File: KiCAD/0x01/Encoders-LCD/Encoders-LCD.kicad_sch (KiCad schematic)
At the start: 32 parts, among them J1 Conn_01x04, J2 Conn_01x04, SW1 SW_LEFT, SW2 SW_SHIFT, SW3 SW_RIGHT, U1 ATtiny412-SS, U2 3631AS, U3 3631AS, U4 ATtiny412-SS, U5 HT16K33 24SOP, U6 ATtiny412-SS

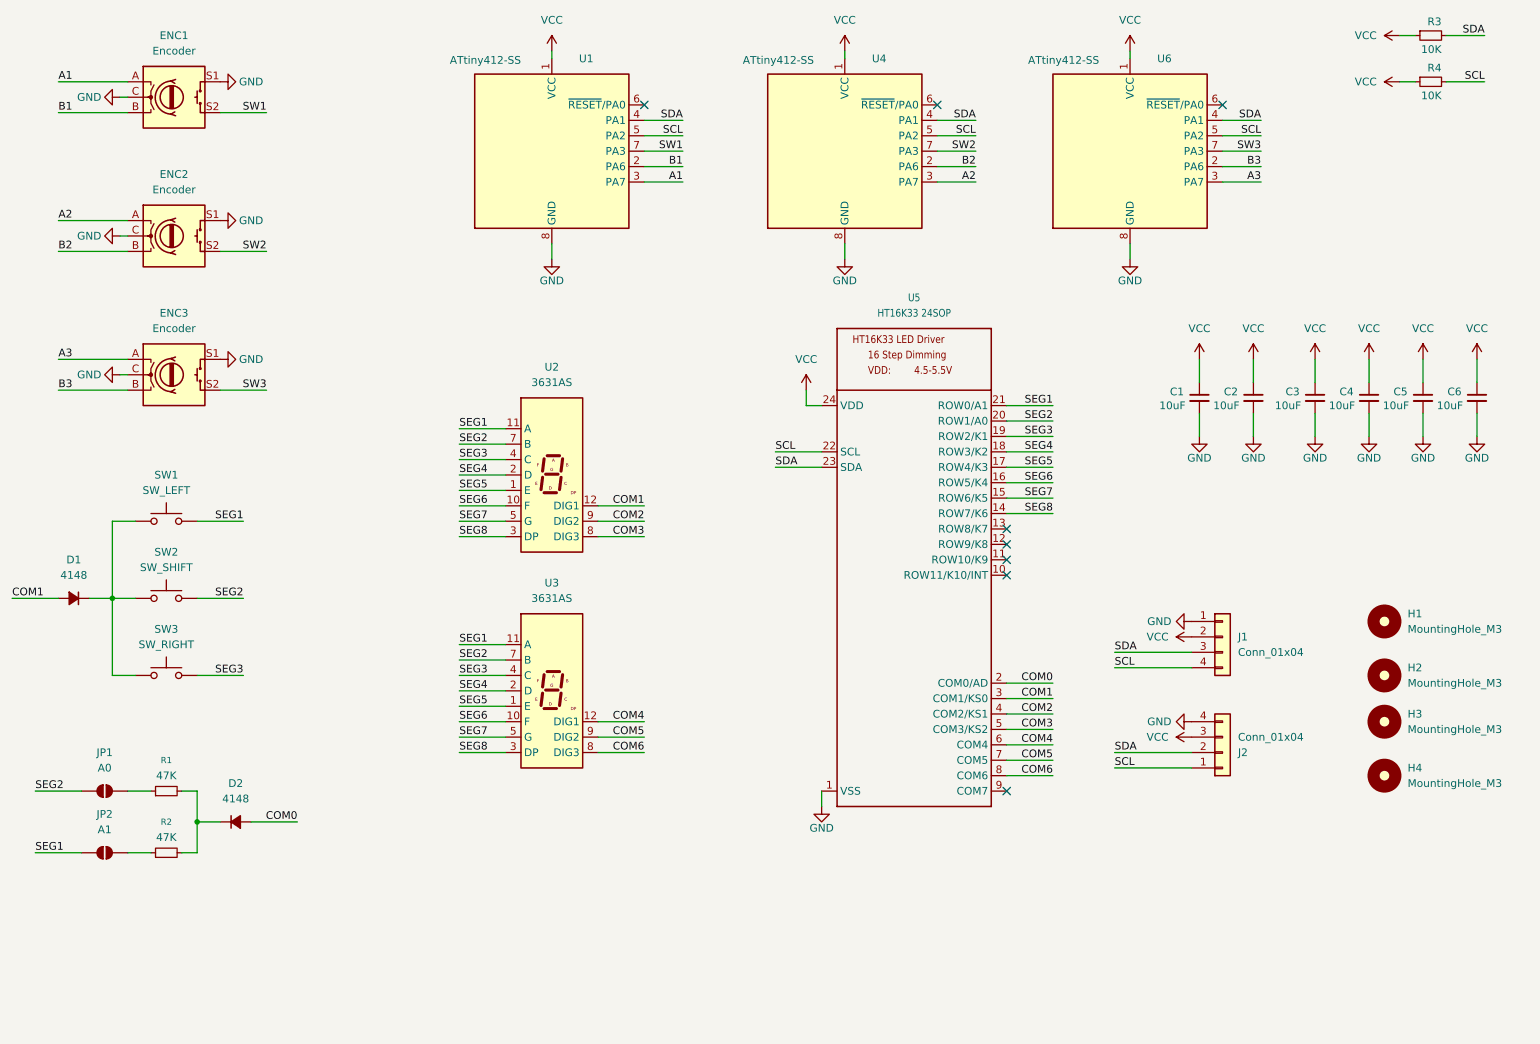
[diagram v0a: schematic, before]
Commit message: lcd encoders
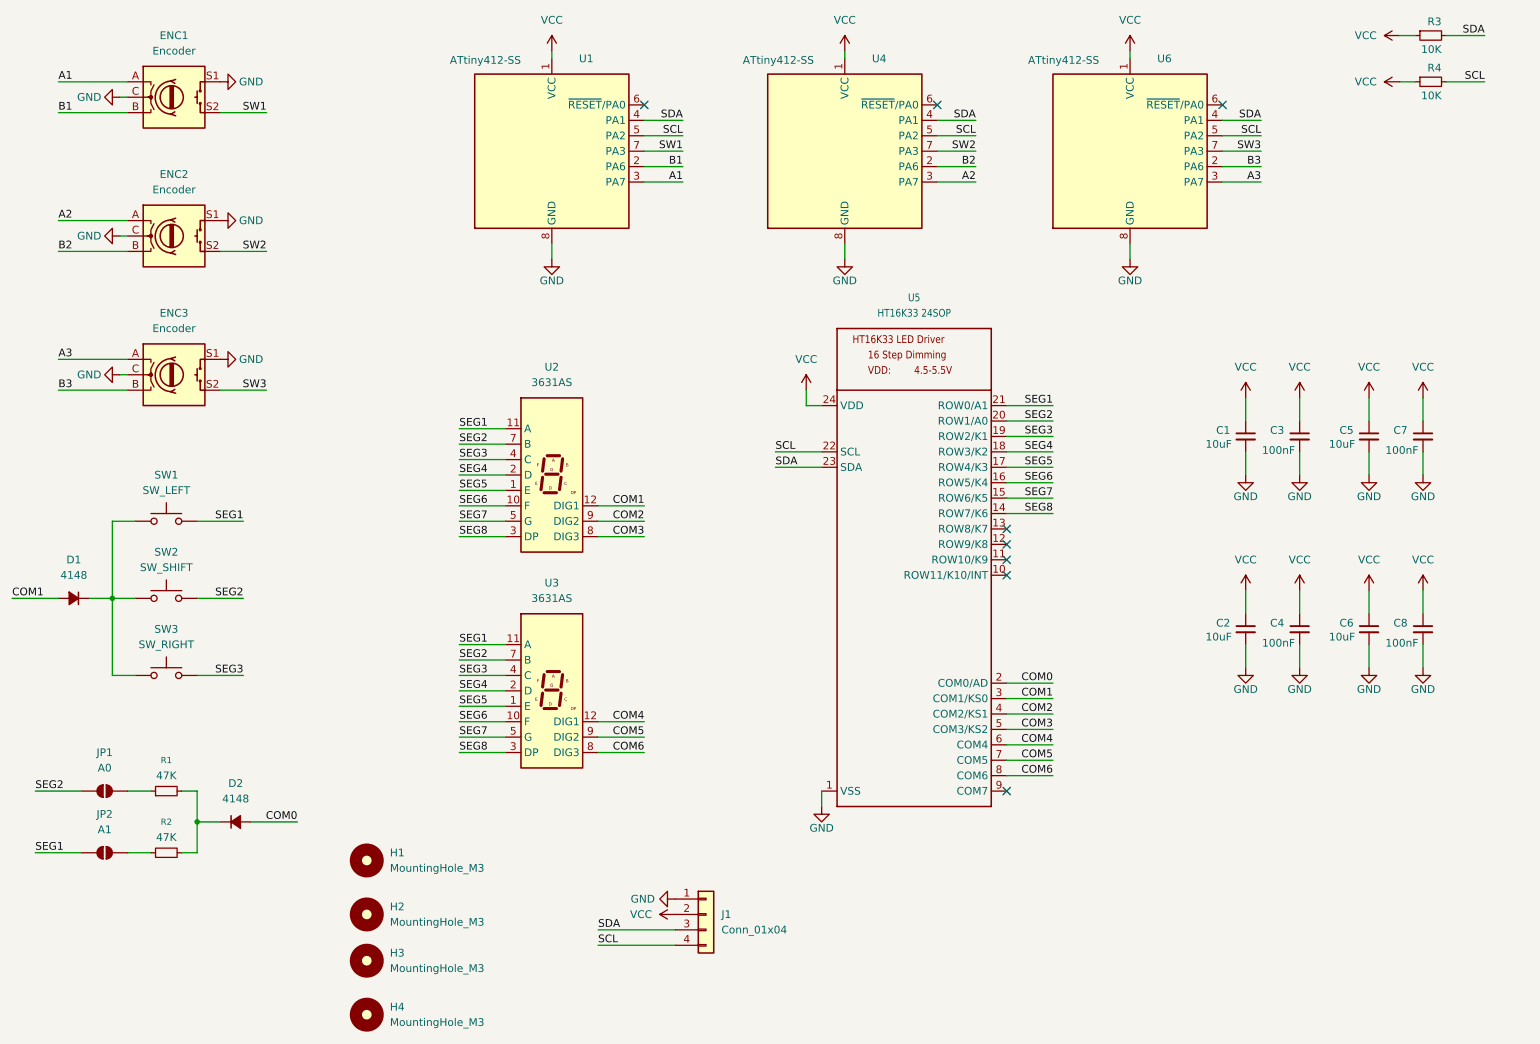
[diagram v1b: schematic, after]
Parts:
- removed C3: 10uF, Capacitor_SMD:C_0805_2012Metric_Pad1.18x1.45mm_HandSolder, symbol Device:C_Small
- removed J2: Conn_01x04, Connector_JST:JST_PH_S4B-PH-K_1x04_P2.00mm_Horizontal, symbol Connector_Generic:Conn_01x04
- added C2: 10uF, Capacitor_SMD:C_0805_2012Metric_Pad1.18x1.45mm_HandSolder, symbol Device:C_Small
- added C7, C8: 100nF, Capacitor_SMD:C_0603_1608Metric_Pad1.08x0.95mm_HandSolder, symbol Device:C_Small
- C3: renamed from C2; value 10uF -> 100nF; footprint Capacitor_SMD:C_0805_2012Metric_Pad1.18x1.45mm_HandSolder -> Capacitor_SMD:C_0603_1608Metric_Pad1.08x0.95mm_HandSolder
- C4: value 10uF -> 100nF; footprint Capacitor_SMD:C_0805_2012Metric_Pad1.18x1.45mm_HandSolder -> Capacitor_SMD:C_0603_1608Metric_Pad1.08x0.95mm_HandSolder
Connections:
- net GND: now also C2.2, C7.2, C8.2
- net VCC: now also C2.1, C7.1, C8.1
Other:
- moved on the sheet: C1, C3, H1, H2, H3, H4, J1
